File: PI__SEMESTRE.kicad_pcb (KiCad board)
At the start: 2 copper layers, 32 parts, among them IC1 LMV358IDR, J1 CX90B-16P1, U1 AMS1117, U11 ESP32-S3-WROOM-1, U14 BME688, U9 GUVA-S12SD

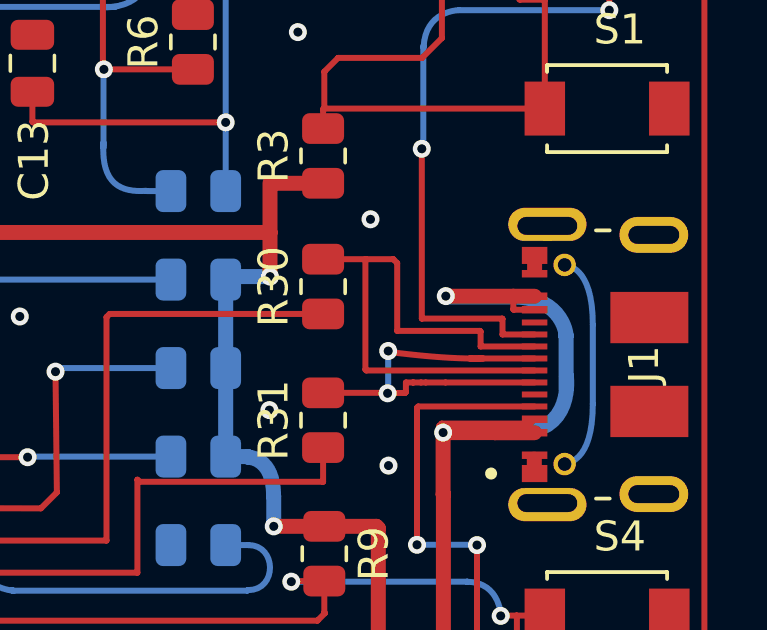
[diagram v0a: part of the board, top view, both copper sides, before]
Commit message: ignorar
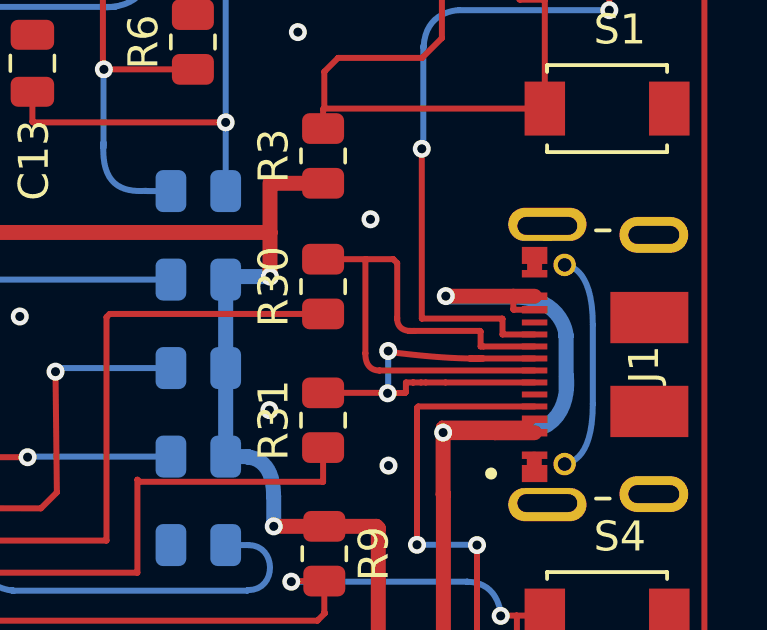
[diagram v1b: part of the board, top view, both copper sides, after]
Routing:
- net D-: track 19.2 -> 17.4 mm
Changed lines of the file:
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@@
+	(gr_curve
+		(pts
+			(xy 117.66 77.79) (xy 117.66 77.79) (xy 117.66 77.79) (xy 117.66 77.79)
+		)
+		(stroke
+			(width 0.2)
+			(type default)
+		)
+		(layer "F.Cu")
+	)
+	(gr_curve
+		(pts
+			(xy 117.78 78.16) (xy 117.78 78.16) (xy 117.78 78.16) (xy 117.78 78.16)
+		)
+		(stroke
+			(width 0.2)
+			(type default)
+		)
+		(layer "F.Cu")
+	)
+	(gr_curve
+		(pts
+			(xy 117.95 78.16) (xy 117.95 78.16) (xy 117.95 78.16) (xy 117.95 78.16)
+		)
+		(stroke
+			(width 0.2)
+			(type default)
+		)
+		(layer "F.Cu")
+	)
+	(gr_curve
+		(pts
+			(xy 118.132243 78.36) (xy 118.13 78.36) (xy 117.63 78.41) (xy 117.65 77.78)
+		)
+		(stroke
+			(width 0.2)
+			(type default)
+		)
+		(layer "F.Cu")
+		(net "D-")
+	)
+	(gr_curve
+		(pts
+			(xy 119.28 77.04) (xy 119.1 77.06) (xy 118.69 77.04) (xy 118.711185 76.600764)
+		)
+		(stroke
+			(width 0.2)
+			(type default)
+		)
+		(layer "F.Cu")
+		(net "D-")
+	)
 	(gr_curve
 		(pts
@@
 	)
 	(segment
-		(start 121.49 77.56)
-		(end 123.29 77.56)
+		(start 118.71 76.64)
+		(end 118.71 74.78)
+		(width 0.2)
+		(layer "F.Cu")
+		(net "D-")
+	)
+	(segment
+		(start 121.49 77.06)
+		(end 121.47 77.04)
+		(width 0.2)
+		(layer "F.Cu")
+		(net "D-")
+	)
+	(segment
+		(start 123.29 78.36)
+		(end 118.11 78.36)
+		(width 0.2)
+		(layer "F.Cu")
+		(net "D-")
+	)
+	(segment
+		(start 118.58 74.65)
+		(end 117.66 74.65)
+		(width 0.2)
+		(layer "F.Cu")
+		(net "D-")
+	)
+	(segment
+		(start 117.65 74.66)
+		(end 117.66 74.65)
+		(width 0.2)
+		(layer "F.Cu")
+		(net "D-")
+	)
+	(segment
+		(start 123.29 77.56)
+		(end 121.581281 77.56)
+		(width 0.2)
+		(layer "F.Cu")
+		(net "D-")
+	)
+	(segment
+		(start 121.49 77.559449)
+		(end 121.49 77.06)
+		(width 0.2)
+		(layer "F.Cu")
+		(net "D-")
+	)
+	(segment
+		(start 121.581281 77.56)
+		(end 121.49 77.559449)
+		(width 0.2)
+		(layer "F.Cu")
+		(net "D-")
+	)
+	(segment
+		(start 117.65 77.79)
+		(end 117.65 74.66)
+		(width 0.2)
+		(layer "F.Cu")
+		(net "D-")
+	)
+	(segment
+		(start 121.47 77.04)
+		(end 119.11 77.04)
+		(width 0.2)
+		(layer "F.Cu")
+		(net "D-")
+	)
+	(segment
+		(start 117.66 74.65)
+		(end 116.24 74.65)
 		(width 0.2)
 		(layer "F.Cu")
@@
 		(width 0.2)
 		(layer "F.Cu")
-		(net "D-")
-	)
-	(segment
-		(start 118.71 77.04)
-		(end 118.71 74.78)
-		(width 0.2)
-		(layer "F.Cu")
-		(net "D-")
-	)
-	(segment
-		(start 117.65 78.33)
-		(end 117.65 74.66)
-		(width 0.2)
-		(layer "F.Cu")
-		(net "D-")
-	)
-	(segment
-		(start 117.68 78.36)
-		(end 117.65 78.33)
-		(width 0.2)
-		(layer "F.Cu")
-		(net "D-")
-	)
-	(segment
-		(start 117.65 74.66)
-		(end 117.66 74.65)
-		(width 0.2)
-		(layer "F.Cu")
-		(net "D-")
-	)
-	(segment
-		(start 118.58 74.65)
-		(end 117.66 74.65)
-		(width 0.2)
-		(layer "F.Cu")
-		(net "D-")
-	)
-	(segment
-		(start 123.29 78.36)
-		(end 117.68 78.36)
-		(width 0.2)
-		(layer "F.Cu")
-		(net "D-")
-	)
-	(segment
-		(start 118.71 77.04)
-		(end 121.47 77.04)
-		(width 0.2)
-		(layer "F.Cu")
-		(net "D-")
-	)
-	(segment
-		(start 121.47 77.04)
-		(end 121.49 77.06)
-		(width 0.2)
-		(layer "F.Cu")
-		(net "D-")
-	)
-	(segment
-		(start 117.66 74.65)
-		(end 116.24 74.65)
-		(width 0.2)
-		(layer "F.Cu")
-		(net "D-")
-	)
-	(segment
-		(start 121.49 77.06)
-		(end 121.49 77.56)
-		(width 0.2)
-		(layer "F.Cu")
